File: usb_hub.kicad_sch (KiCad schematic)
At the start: 2 parts, among them J2 D-SUB 9 Male

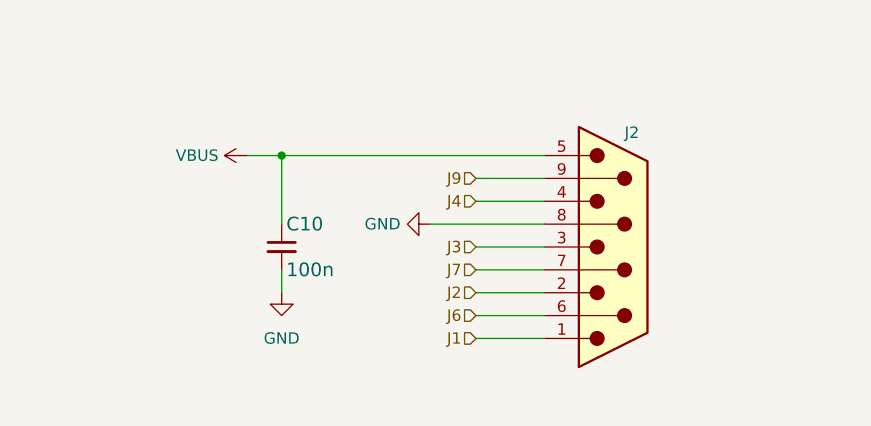
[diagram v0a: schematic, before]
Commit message: Minor fixes
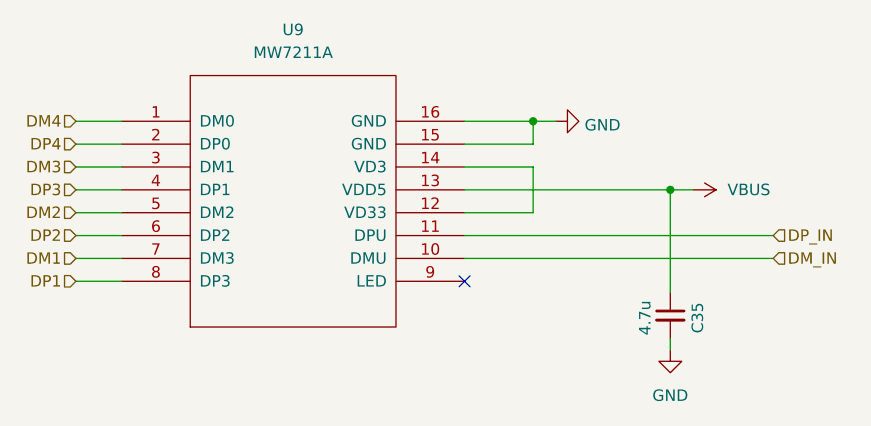
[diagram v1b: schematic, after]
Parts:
- removed C10: 100n, FRANK:Capacitor (0805), symbol Device:C_Small
- removed J2: D-SUB 9 Male, FRANK:D-SUB (9 pin, male, top mount), symbol FRANK:DB9_Male_Small
- added C35: 4.7u, FRANK:Capacitor (0805), symbol Device:C_Small
- added U9: MW7211A, FRANK:SOP-16, symbol FRANK:MW7211A
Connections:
- net GND: now also C35.2, U9.15 (GND), U9.16 (GND)
- net VBUS: now also C35.1, U9.13 (VDD5)
- new net: U9.12 (VD33), U9.14 (VD3)
- new net DM1: U9.7 (DM3)
- new net DM2: U9.5 (DM2)
- new net DM3: U9.3 (DM1)
- new net DM4: U9.1 (DM0)
- new net DM_IN: U9.10 (DMU)
- new net DP1: U9.8 (DP3)
- new net DP2: U9.6 (DP2)
- new net DP3: U9.4 (DP1)
- new net DP4: U9.2 (DP0)
- new net DP_IN: U9.11 (DPU)
- no-connect marks 0 -> 1
